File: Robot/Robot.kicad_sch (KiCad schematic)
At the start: 1 part

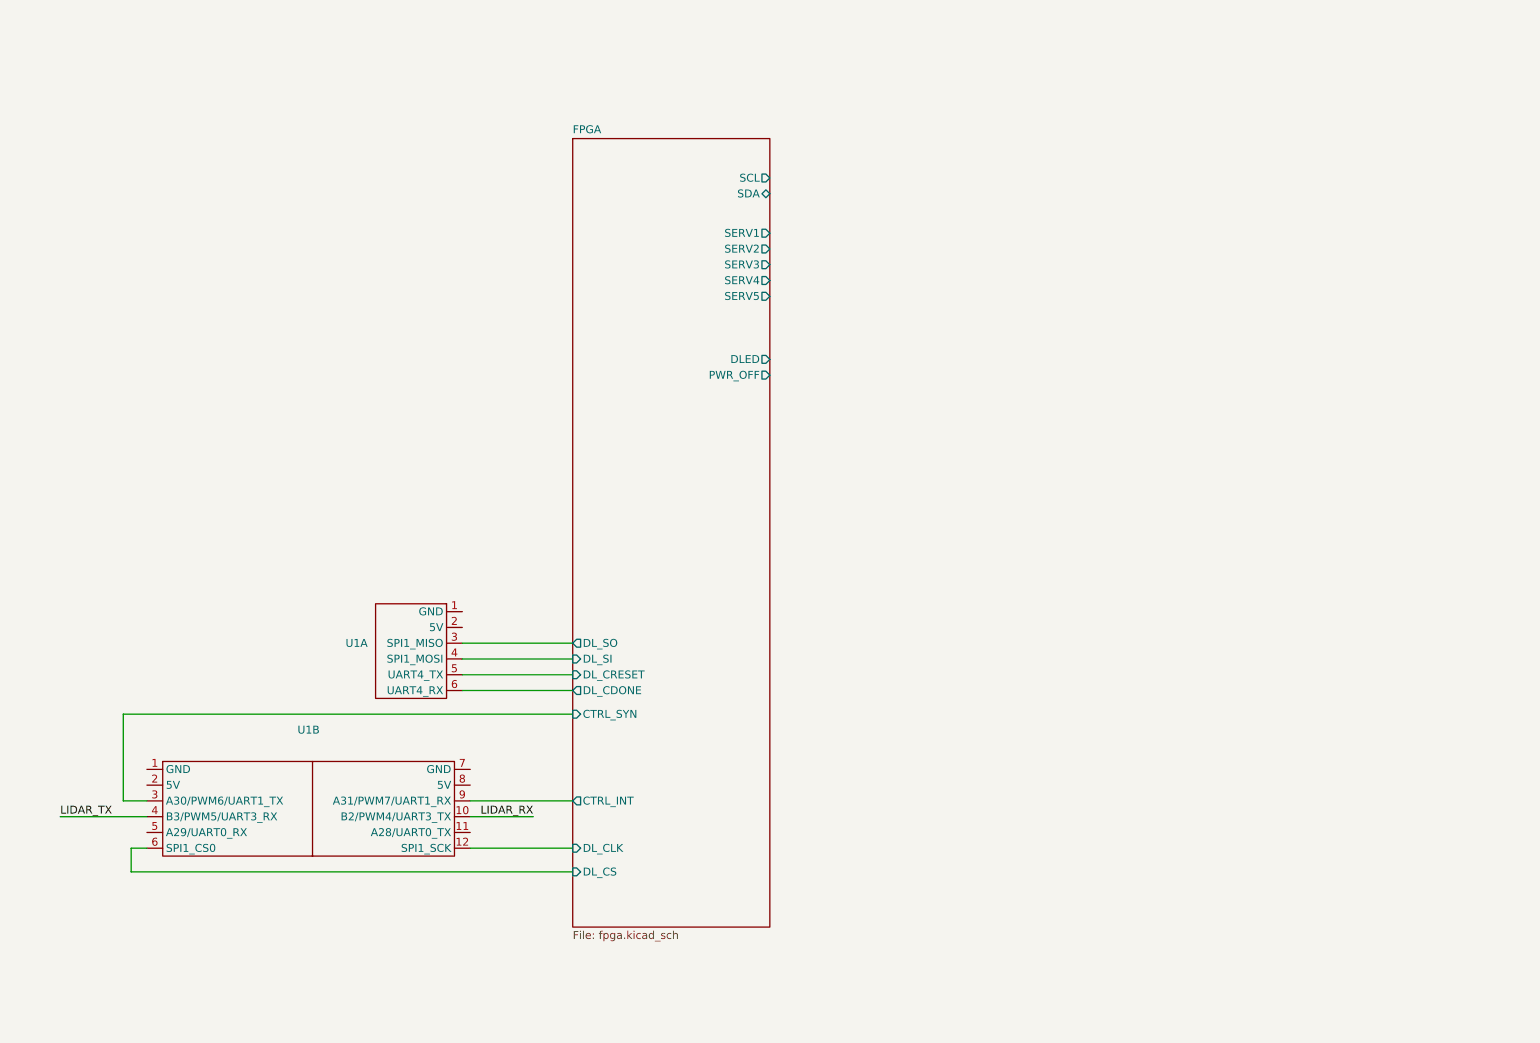
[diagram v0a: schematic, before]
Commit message: Updated Robot SCH
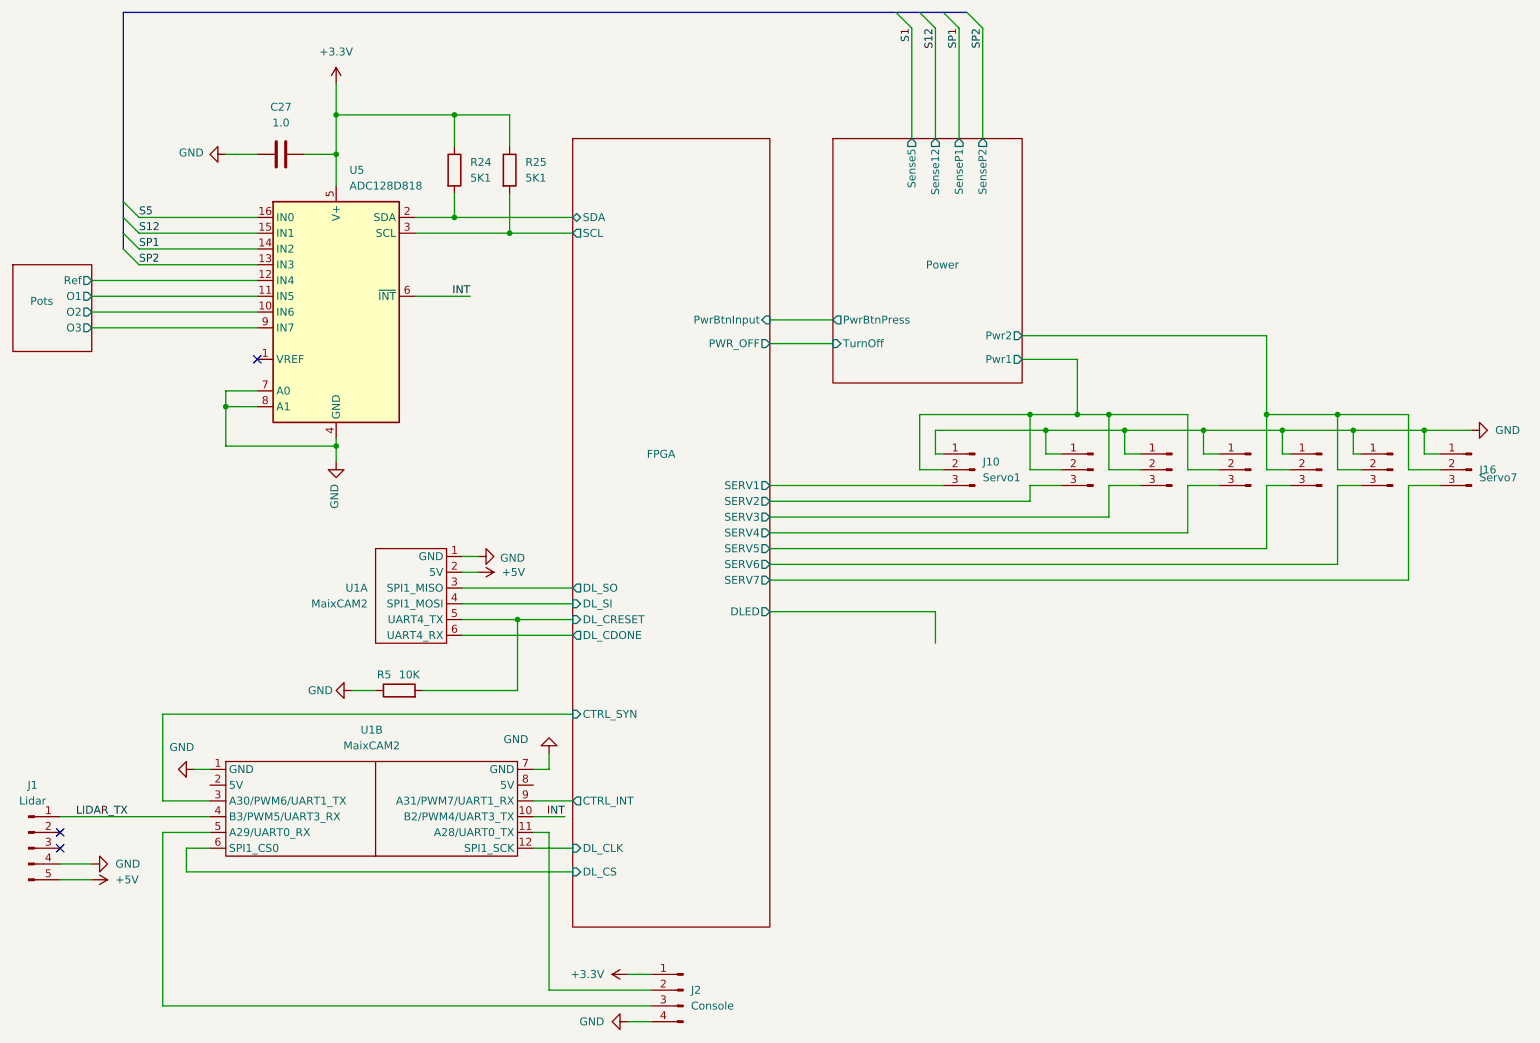
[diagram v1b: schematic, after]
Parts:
- added C27: 1.0, symbol Device:C
- added J1: Lidar, symbol Connector:Conn_01x05_Pin
- added J10: Servo1, symbol Connector:Conn_01x03_Pin
- added J11: Servo2, symbol Connector:Conn_01x03_Pin
- added J12: Servo3, symbol Connector:Conn_01x03_Pin
- added J13: Servo4, symbol Connector:Conn_01x03_Pin
- added J14: Servo5, symbol Connector:Conn_01x03_Pin
- added J15: Servo6, symbol Connector:Conn_01x03_Pin
- added J16: Servo7, symbol Connector:Conn_01x03_Pin
- added J2: Console, symbol Connector:Conn_01x04_Pin
- added R24, R25: 5K1, symbol Device:R
- added R5: 10K, Resistor_SMD:R_0603_1608Metric_Pad0.98x0.95mm_HandSolder, symbol Device:R
- added U5: ADC128D818, Package_SO:TSSOP-16_4.4x5mm_P0.65mm, symbol Analog_ADC:ADC128D818
- U1: value ~ -> MaixCAM2
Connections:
- net FPGA/DL_CRESET: now also R5.2
- net FPGA/SCL: now also R25.2, U5.3 (SCL)
- net FPGA/SDA: now also R24.2, U5.2 (SDA)
- net FPGA/SERV1: now also J10.3 (Pin_3)
- net FPGA/SERV2: now also J11.3 (Pin_3)
- net FPGA/SERV3: now also J12.3 (Pin_3)
- net FPGA/SERV4: now also J13.3 (Pin_3)
- net FPGA/SERV5: now also J14.3 (Pin_3)
- net LIDAR_TX: now also J1.1 (Pin_1)
- net GND: now reaches U1.1 (GND)
- net GND: now also U1.1 (GND), U1.7 (GND), C27.1, J1.4 (Pin_4), J10.1 (Pin_1), J11.1 (Pin_1), J12.1 (Pin_1), J13.1 (Pin_1), J14.1 (Pin_1), J15.1 (Pin_1), J16.1 (Pin_1), J2.4 (Pin_4), R5.1, U5.4 (GND), U5.7 (A0), U5.8 (A1)
- net +5V: now reaches U1.2 (5V)
- net +5V: now also J1.5 (Pin_5)
- net at U1.11 (A28/UART0_TX): now also J2.2 (Pin_2)
- net at U1.5 (A29/UART0_RX): now also J2.3 (Pin_3)
- net LIDAR_RX renamed INT
- net INT: now also U5.6 (~{INT})
- new net +3.3V: C27.2, J2.1 (Pin_1), R24.1, R25.1, U5.5 (V+)
- new net FPGA/SERV6: J15.3 (Pin_3)
- new net FPGA/SERV7: J16.3 (Pin_3)
- new net Pots/O1: U5.11 (IN5)
- new net Pots/O2: U5.10 (IN6)
- new net Pots/O3: U5.9 (IN7)
- new net Pots/Ref: U5.12 (IN4)
- new net Power/Pwr1: J10.2 (Pin_2), J11.2 (Pin_2), J12.2 (Pin_2), J13.2 (Pin_2)
- new net Power/Pwr2: J14.2 (Pin_2), J15.2 (Pin_2), J16.2 (Pin_2)
- new net S12: U5.15 (IN1)
- new net S5: U5.16 (IN0)
- new net SP1: U5.14 (IN2)
- new net SP2: U5.13 (IN3)
- no-connect marks 0 -> 3
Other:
- added sheet Pots (pots.kicad_sch)
- added sheet Power (power.kicad_sch)
- sheet FPGA ports: added PwrBtnInput, SERV6, SERV7; removed none
- moved on the sheet: U1A, U1B
